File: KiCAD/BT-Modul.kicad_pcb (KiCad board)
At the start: 2 copper layers, 63.5 x 63.5 mm, 17 parts, among them P1 CONN_01X03, P2 USB_B, P3 USB_A, U1 KRC-86B, U2 ICL7660S, U3 opa2134

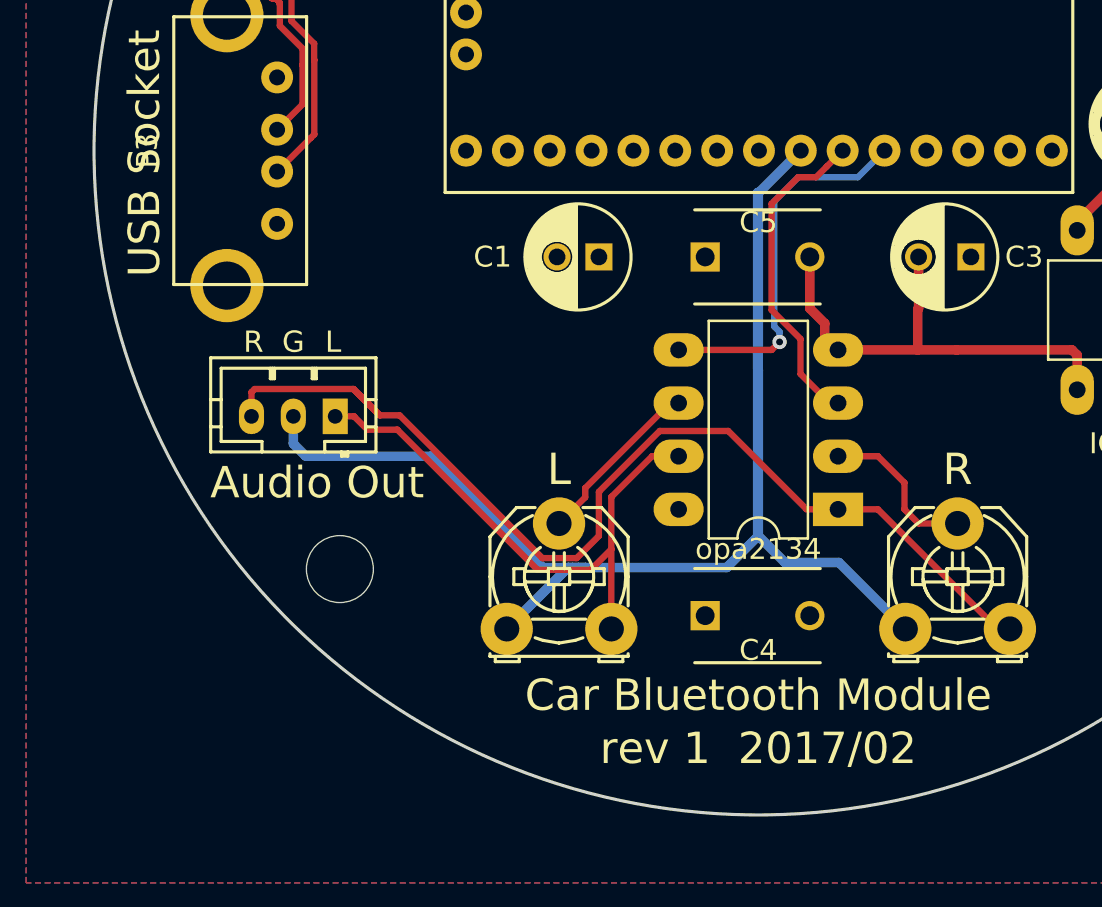
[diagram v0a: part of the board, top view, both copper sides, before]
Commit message: Rev 1 as ordered
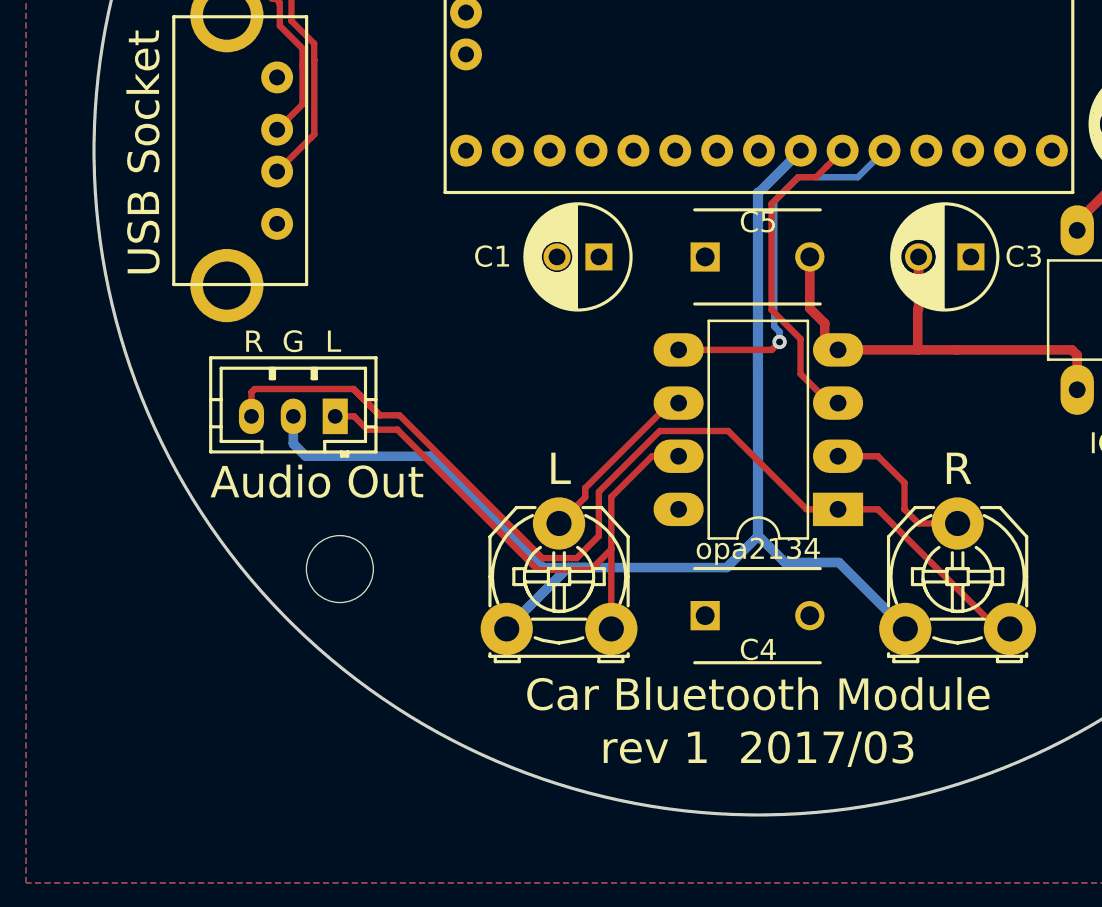
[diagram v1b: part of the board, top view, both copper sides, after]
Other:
- board text added: "rev 1 2017/03"
- board text removed: "rev 1 2017/02"
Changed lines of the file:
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@@
   (module BTA:USB_A_Fem_Vert (layer F.Cu)
     (at 69.6 95 270)
-    (fp_text reference P3 (at 0 3.81 270) (layer F.SilkS)
+    (fp_text reference P3 (at 0 3.81 270) (layer F.SilkS) hide
       (effects (font (size 1 1) (thickness 0.15)))
     )
@@
     (effects (font (size 1.5 1.5) (thickness 0.3)))
   )
-  (gr_text "rev 1  2017/02" (at 95 123.575) (layer F.SilkS)
+  (gr_text "rev 1  2017/03" (at 95 123.575) (layer F.SilkS)
     (effects (font (size 1.5 1.5) (thickness 0.3)))
   )
